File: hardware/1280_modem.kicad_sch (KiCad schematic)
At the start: 88 parts, among them IC1 SX1281IMLTRT, IC2 SKY65383-11, IC3 LMR50410Y3, J2 Conn_Coaxial, J2 jst gh 4, J5 jst gh 6, J8 USB_C_Receptacle_USB2.0, J9 jst_sh 6, Q1 AO3401A, Q2 AO3401A, U13 STM32U575CGTx, U2 TPS7A20285PDBVR, U2 USBLC6-2SC6, U4 TCAN334, Y1 48MHz, Y1 52MHz

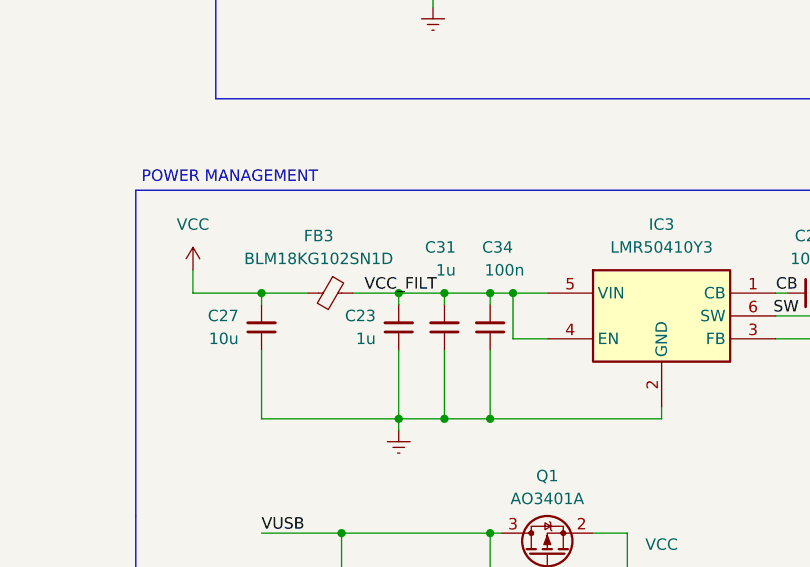
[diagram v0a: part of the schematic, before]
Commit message: bamse
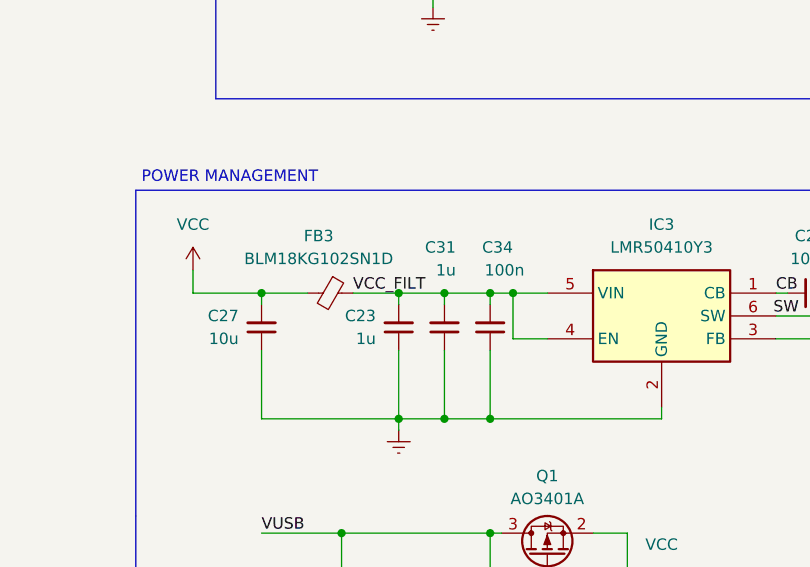
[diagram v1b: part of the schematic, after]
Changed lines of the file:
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@@
     (effects (font (size 1.27 1.27)) (justify right bottom))
   )
-  (label "VCC_FILT" (at 189.23 215.9 0) (fields_autoplaced)
+  (label "VCC_FILT" (at 187.96 215.9 0) (fields_autoplaced)
     (effects (font (size 1.27 1.27)) (justify left bottom))
   )
